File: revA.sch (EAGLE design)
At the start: 23 parts

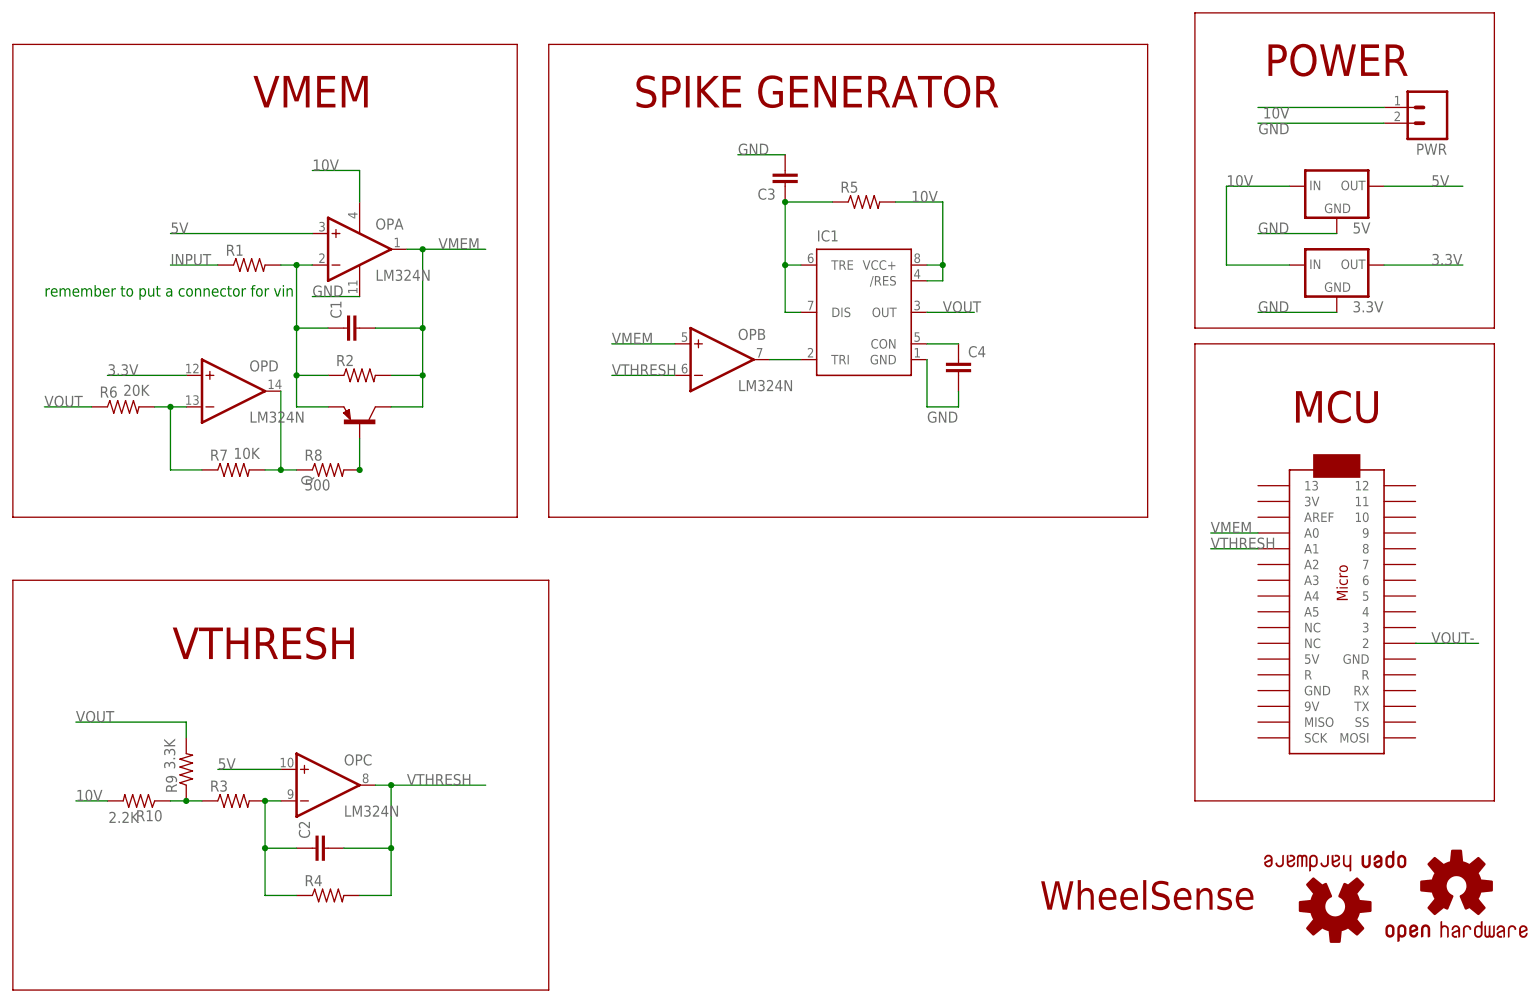
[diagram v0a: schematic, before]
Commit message: revA done
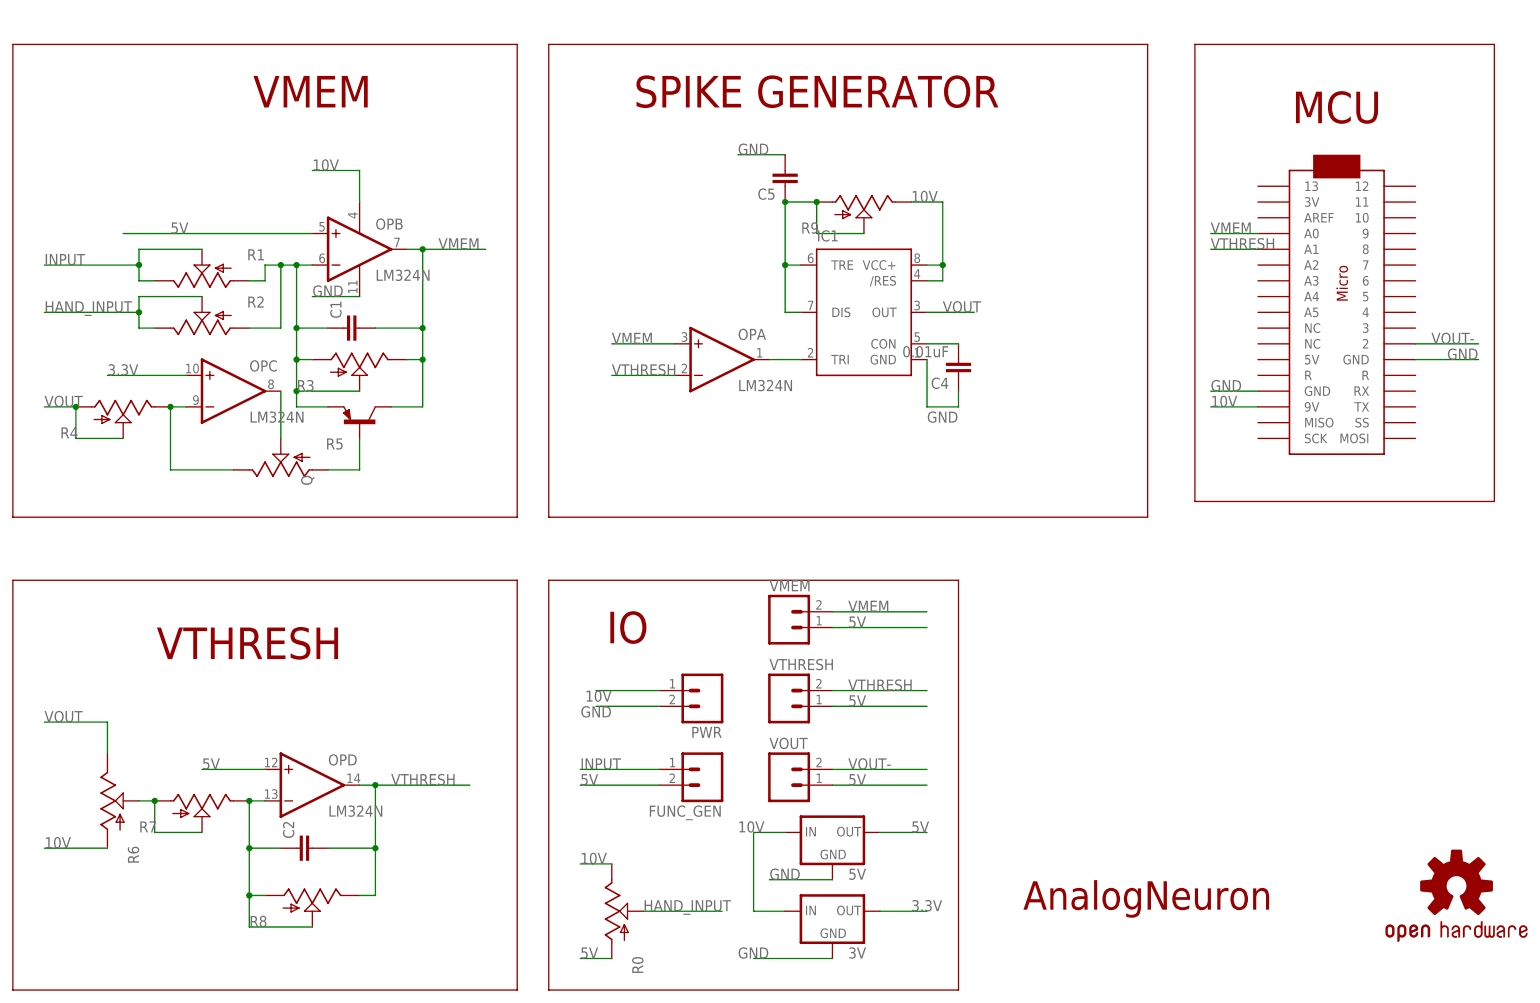
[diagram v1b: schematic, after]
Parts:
- removed 3.3V: (no value), SparkFun-PowerIC:V_REG_78XXSIDE
- removed C3: (no value), SparkFun-Passives:CAPPTH
- removed LOGO2: OSHW-LOGOL-TOP, SparkFun-Aesthetics:OSHW-LOGOL-TOP
- removed R10: 2.2K, SparkFun-Passives:RESISTORPTH-1/4W
- added 3V: (no value), v-reg:78LXX
- added C5: (no value), SparkFun-Passives:CAPPTH1
- added FUNC_GEN, VMEM, VOUT, VTHRESH: (no value), SparkFun-Connectors:M023.5MM
- added R0: (no value), SparkFun-Electromechanical:POT
- 5V: device SparkFun-PowerIC:V_REG_78XXSIDE -> v-reg:78LXX
- C4: value (none) -> 0.01uF; device SparkFun-Passives:CAPPTH -> SparkFun-Passives:CAPPTH1
- R1, R2, R3, R4, R5: device SparkFun-Passives:RESISTORPTH-1/4W -> SparkFun-Electromechanical:POT
- R6: value 20K -> (none); device SparkFun-Passives:RESISTORPTH-1/4W -> SparkFun-Electromechanical:POT
- R7: value 10K -> (none); device SparkFun-Passives:RESISTORPTH-1/4W -> SparkFun-Electromechanical:POT
- R8: value 500 -> (none); device SparkFun-Resistors:RESISTORPTH-1/4W -> SparkFun-Electromechanical:POT
- R9: value 3.3K -> (none); device SparkFun-Passives:RESISTORPTH-1/4W -> SparkFun-Electromechanical:POT
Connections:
- removed net N$3: R10.1, R3.1, R9.1
- new net HAND_INPUT: R0.S, R2.E, R2.S
- new net R7: R6.S, R7.A, R7.S
- net 10V: now also 3V.IN, R0.E, R6.A, R9.E, U$1.9V; no longer 3.3V.IN, R10.2, R5.2
- net 2: now also OPB.-IN, R1.A, R2.A, R3.A, R3.S; no longer OPA.-IN, R1.2, R2.1
- net 3.3V: now also 3V.OUT, OPC.+IN; no longer 3.3V.OUT, OPD.+IN
- net 5V: now also FUNC_GEN.2, OPB.+IN, OPD.+IN, R0.A, VMEM.1, VOUT.1, VTHRESH.1; no longer OPA.+IN, OPC.+IN
- net CON: now also C4.2; no longer C4.1
- net GND: now also 3V.GND, C4.1, C5.2, U$1.GND, U$1.GND@1; no longer 3.3V.GND, C3.2, C4.2
- net INPUT: now also FUNC_GEN.1, R1.E, R1.S; no longer R1.1
- net N$1: now also C5.1, R9.A, R9.S; no longer C3.1, R5.1
- net N$2: now also R5.A; no longer R8.2
- net N$4: now also OPC.-IN, R4.E, R5.E; no longer OPD.-IN, R6.2, R7.1
- net N$9: now also OPD.-IN, R7.E, R8.A, R8.S; no longer OPC.-IN, R3.2, R4.1
- net TRI: now also OPA.OUT; no longer OPB.OUT
- net VMEM: now also OPA.+IN, OPB.OUT, R3.E, VMEM.2; no longer OPA.OUT, OPB.+IN, R2.2
- net VOUT: now also R4.A, R4.S, R6.E; no longer R6.1, R9.2
- net VOUT-: now also OPC.OUT, R5.S, VOUT.2; no longer OPD.OUT, R7.2, R8.1
- net VTHRESH: now also OPA.-IN, OPD.OUT, R8.E, VTHRESH.2; no longer OPB.-IN, OPC.OUT, R4.2
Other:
- note added: "AnalogNeuron"
- note added: "IO"
- note removed: "POWER"
- note removed: "WheelSense"
- note removed: "remember to put a connector for vin"
- moved on the sheet: C2, C4, OPA, OPB, OPC, OPD, PWR
